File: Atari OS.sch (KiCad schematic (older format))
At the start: 3 parts, among them J51 OS Type, U7 27C512

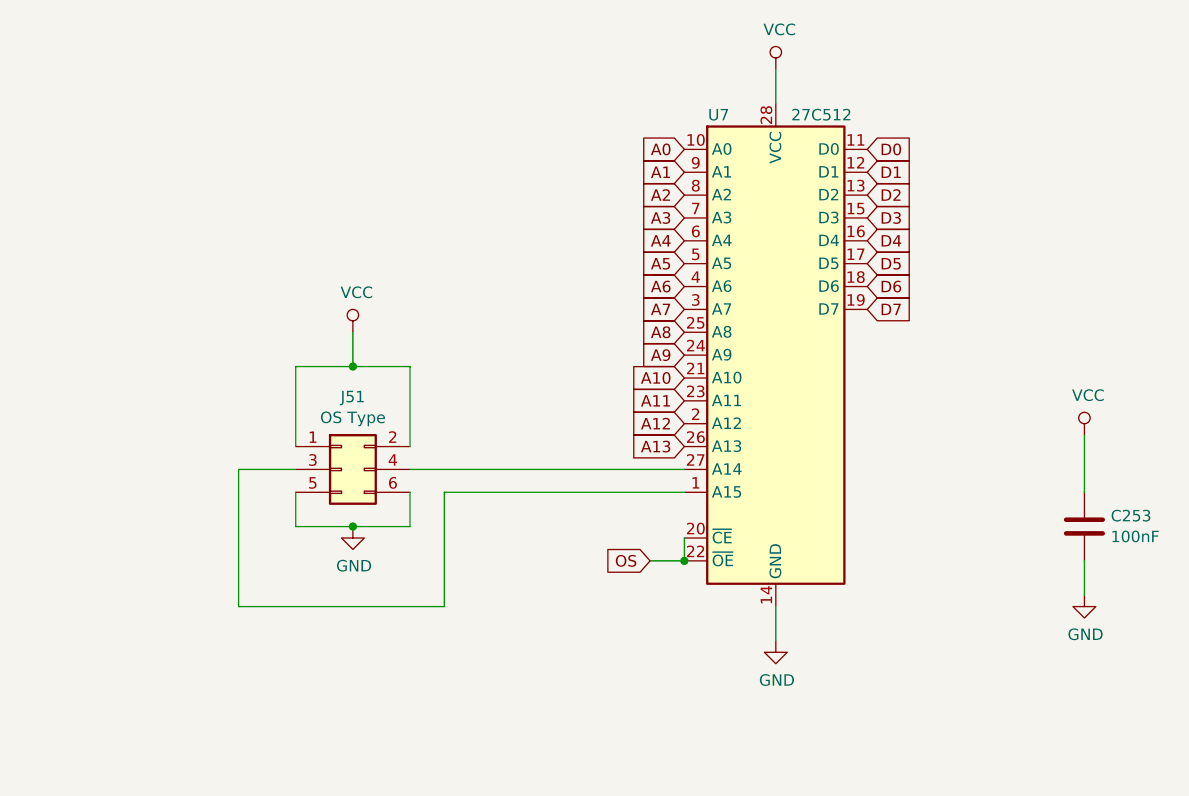
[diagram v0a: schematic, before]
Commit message: Track OS and Basic
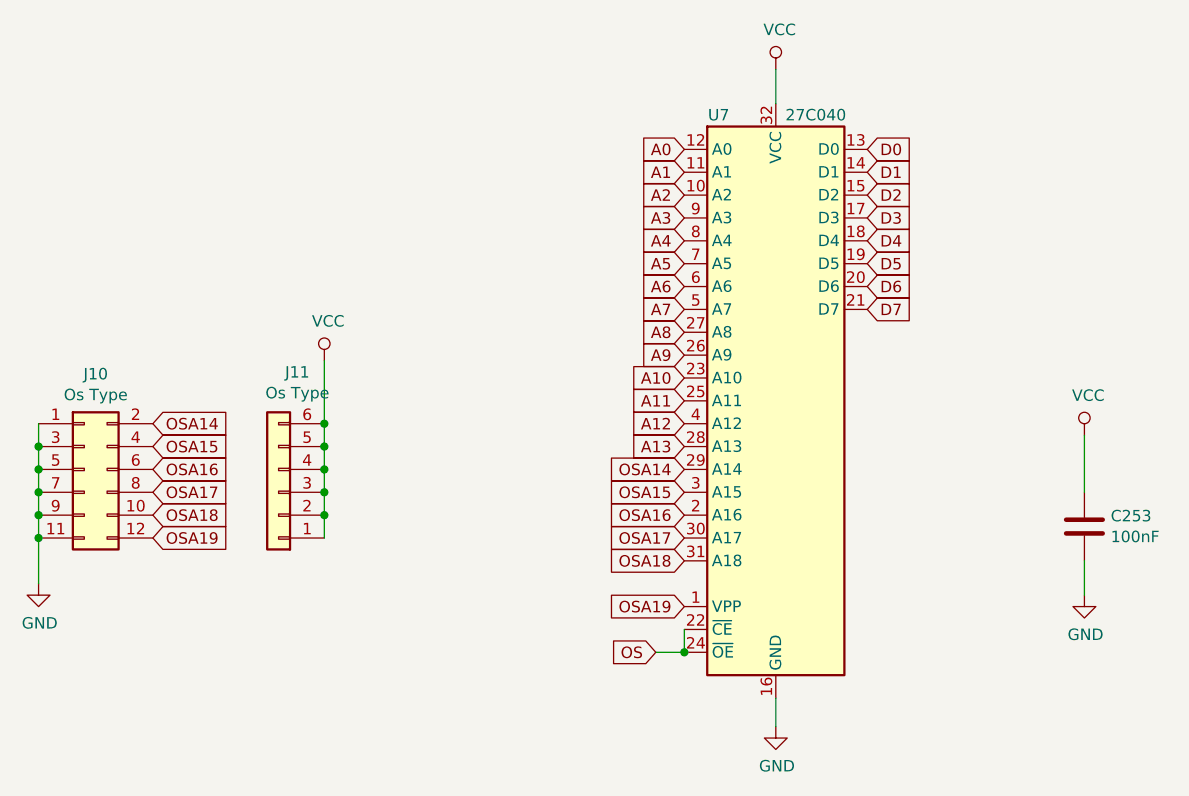
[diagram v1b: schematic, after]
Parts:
- removed J51: OS Type, Connector_PinHeader_2.54mm:PinHeader_2x03_P2.54mm_Vertical, symbol Connector_Generic:Conn_02x03_Odd_Even
- removed U7: 27C512, Package_DIP:DIP-28_W15.24mm_LongPads, symbol Memory_EPROM:27C512
- added J10: Os Type, Connector_PinHeader_2.54mm:PinHeader_2x06_P2.54mm_Vertical, symbol Connector_Generic:Conn_02x06_Odd_Even
- added J11: Os Type, Connector_PinHeader_2.54mm:PinHeader_1x06_P2.54mm_Vertical, symbol Connector_Generic:Conn_01x06
- added U7: 27C040, Package_DIP:DIP-32_W15.24mm_Socket_LongPads, symbol Memory_EPROM:27C040
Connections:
- net A0: now also U7.12 (A0)
- net A1: now also U7.11 (A1)
- net A10: now also U7.23 (A10)
- net A11: now also U7.25 (A11)
- net A12: now also U7.4 (A12)
- net A13: now also U7.28 (A13)
- net A2: now also U7.10 (A2)
- net A3: now also U7.9 (A3)
- net A4: now also U7.8 (A4)
- net A5: now also U7.7 (A5)
- net A6: now also U7.6 (A6)
- net A7: now also U7.5 (A7)
- net A8: now also U7.27 (A8)
- net A9: now also U7.26 (A9)
- net D0: now also U7.13 (D0)
- net D1: now also U7.14 (D1)
- net D2: now also U7.15 (D2)
- net D3: now also U7.17 (D3)
- net D4: now also U7.18 (D4)
- net D5: now also U7.19 (D5)
- net D6: now also U7.20 (D6)
- net D7: now also U7.21 (D7)
- net GND: now also J10.1 (Pin_1), J10.11 (Pin_11), J10.3 (Pin_3), J10.5 (Pin_5), J10.7 (Pin_7), J10.9 (Pin_9), U7.16 (GND)
- net OS: now also U7.22 (~CE), U7.24 (~OE)
- net VCC: now also J11.1 (Pin_1), J11.2 (Pin_2), J11.3 (Pin_3), J11.4 (Pin_4), J11.5 (Pin_5), J11.6 (Pin_6), U7.32 (VCC)
- new net OSA14: J10.2 (Pin_2), U7.29 (A14)
- new net OSA15: J10.4 (Pin_4), U7.3 (A15)
- new net OSA16: J10.6 (Pin_6), U7.2 (A16)
- new net OSA17: J10.8 (Pin_8), U7.30 (A17)
- new net OSA18: J10.10 (Pin_10), U7.31 (A18)
- new net OSA19: J10.12 (Pin_12), U7.1 (VPP)
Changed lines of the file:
@@
 $EndDescr
-$Comp
-L Memory_EPROM:27C512 U7
-U 1 1 5E64FA8C
-P 5850 3550
-F 0 "U7" H 5600 4600 50  0000 C CNN
-F 1 "27C512" H 6050 4600 50  0000 C CNN
-F 2 "Package_DIP:DIP-28_W15.24mm_LongPads" H 5850 3550 50  0001 C CNN
-F 3 "http://ww1.microchip.com/downloads/en/DeviceDoc/doc0015.pdf" H 5850 3550 50  0001 C CNN
-	1    5850 3550
-	1    0    0    -1
-$EndComp
 $Comp
 L power:VCC #PWR0185
@@
 L power:GND #PWR0186
 U 1 1 5E6514FE
-P 5850 4800
-F 0 "#PWR0186" H 5850 4550 50  0001 C CNN
-F 1 "GND" H 5855 4627 50  0000 C CNN
-F 2 "" H 5850 4800 50  0001 C CNN
-F 3 "" H 5850 4800 50  0001 C CNN
-	1    5850 4800
-	1    0    0    -1
-$EndComp
-Wire Wire Line
-	5850 4650 5850 4800
+P 5850 5175
+F 0 "#PWR0186" H 5850 4925 50  0001 C CNN
+F 1 "GND" H 5855 5002 50  0000 C CNN
+F 2 "" H 5850 5175 50  0001 C CNN
+F 3 "" H 5850 5175 50  0001 C CNN
+	1    5850 5175
+	1    0    0    -1
+$EndComp
 Text GLabel 6250 2650 2    50   Input ~ 0
 D0
@@
 A13
 $Comp
-L Connector_Generic:Conn_02x03_Odd_Even J51
-U 1 1 5E656178
-P 3950 4050
-F 0 "J51" H 4000 4367 50  0000 C CNN
-F 1 "OS Type" H 4000 4276 50  0000 C CNN
-F 2 "Connector_PinHeader_2.54mm:PinHeader_2x03_P2.54mm_Vertical" H 3950 4050 50  0001 C CNN
-F 3 "~" H 3950 4050 50  0001 C CNN
-	1    3950 4050
-	1    0    0    -1
-$EndComp
-$Comp
 L power:GND #PWR0187
 U 1 1 5E6585C8
-P 4000 4300
-F 0 "#PWR0187" H 4000 4050 50  0001 C CNN
-F 1 "GND" H 4005 4127 50  0000 C CNN
-F 2 "" H 4000 4300 50  0001 C CNN
-F 3 "" H 4000 4300 50  0001 C CNN
-	1    4000 4300
-	1    0    0    -1
-$EndComp
-Wire Wire Line
-	3750 4150 3750 4300
-Wire Wire Line
-	3750 4300 4000 4300
-Wire Wire Line
-	4250 4150 4250 4300
-Wire Wire Line
-	4250 4300 4000 4300
-Connection ~ 4000 4300
-Wire Wire Line
-	3750 3950 3750 3600
-Wire Wire Line
-	3750 3600 4000 3600
-Wire Wire Line
-	4250 3600 4250 3950
+P 2625 4550
+F 0 "#PWR0187" H 2625 4300 50  0001 C CNN
+F 1 "GND" H 2630 4377 50  0000 C CNN
+F 2 "" H 2625 4550 50  0001 C CNN
+F 3 "" H 2625 4550 50  0001 C CNN
+	1    2625 4550
+	1    0    0    -1
+$EndComp
 $Comp
 L power:VCC #PWR0188
 U 1 1 5E659359
-P 4000 3450
-F 0 "#PWR0188" H 4000 3300 50  0001 C CNN
-F 1 "VCC" H 4017 3623 50  0000 C CNN
-F 2 "" H 4000 3450 50  0001 C CNN
-F 3 "" H 4000 3450 50  0001 C CNN
-	1    4000 3450
-	1    0    0    -1
-$EndComp
-Wire Wire Line
-	4000 3450 4000 3600
-Connection ~ 4000 3600
-Wire Wire Line
-	4000 3600 4250 3600
-Wire Wire Line
-	5450 4050 4250 4050
-Wire Wire Line
-	5450 4150 4400 4150
-Wire Wire Line
-	4400 4150 4400 4650
-Wire Wire Line
-	4400 4650 3500 4650
-Wire Wire Line
-	3500 4650 3500 4050
-Wire Wire Line
-	3500 4050 3750 4050
-Wire Wire Line
-	5450 4350 5450 4450
-Text GLabel 5300 4450 0    50   Input ~ 0
+P 3875 3575
+F 0 "#PWR0188" H 3875 3425 50  0001 C CNN
+F 1 "VCC" H 3892 3748 50  0000 C CNN
+F 2 "" H 3875 3575 50  0001 C CNN
+F 3 "" H 3875 3575 50  0001 C CNN
+	1    3875 3575
+	1    0    0    -1
+$EndComp
+Text GLabel 5325 4850 0    50   Input ~ 0
 OS
-Wire Wire Line
-	5450 4450 5300 4450
-Connection ~ 5450 4450
 $Comp
 L Device:C C253
@@
 Wire Wire Line
 	7200 3900 7200 4150
+$Comp
+L Memory_EPROM:27C040 U7
+U 1 1 5FC01AF4
+P 5850 3750
+F 0 "U7" H 5600 5000 50  0000 C CNN
+F 1 "27C040" H 6025 5000 50  0000 C CNN
+F 2 "Package_DIP:DIP-32_W15.24mm_Socket_LongPads" H 5850 3750 50  0001 C CNN
+F 3 "http://ww1.microchip.com/downloads/en/devicedoc/doc0189.pdf" H 5850 3750 50  0001 C CNN
+	1    5850 3750
+	1    0    0    -1
+$EndComp
+Wire Wire Line
+	5450 4750 5450 4850
+Wire Wire Line
+	5450 4850 5325 4850
+Connection ~ 5450 4850
+Wire Wire Line
+	5850 5050 5850 5175
+$Comp
+L Connector_Generic:Conn_02x06_Odd_Even J10
+U 1 1 5FC22FF9
+P 2825 4050
+F 0 "J10" H 2875 4467 50  0000 C CNN
+F 1 "Os Type" H 2875 4376 50  0000 C CNN
+F 2 "Connector_PinHeader_2.54mm:PinHeader_2x06_P2.54mm_Vertical" H 2825 4050 50  0001 C CNN
+F 3 "~" H 2825 4050 50  0001 C CNN
+	1    2825 4050
+	1    0    0    -1
+$EndComp
+$Comp
+L Connector_Generic:Conn_01x06 J11
+U 1 1 5FC26BAD
+P 3675 4150
+F 0 "J11" H 3593 3625 50  0000 C CNN
+F 1 "Os Type" H 3593 3716 50  0000 C CNN
+F 2 "Connector_PinHeader_2.54mm:PinHeader_1x06_P2.54mm_Vertical" H 3675 4150 50  0001 C CNN
+F 3 "~" H 3675 4150 50  0001 C CNN
+	1    3675 4150
+	-1   0    0    1
+$EndComp
+Wire Wire Line
+	2625 3850 2625 3950
+Wire Wire Line
+	2625 3950 2625 4050
+Connection ~ 2625 3950
+Wire Wire Line
+	2625 4050 2625 4150
+Connection ~ 2625 4050
+Wire Wire Line
+	2625 4150 2625 4250
+Connection ~ 2625 4150
+Wire Wire Line
+	2625 4250 2625 4350
+Connection ~ 2625 4250
+Wire Wire Line
+	2625 4350 2625 4550
+Connection ~ 2625 4350
+Wire Wire Line
+	3875 3850 3875 3950
+Wire Wire Line
+	3875 4050 3875 3950
+Connection ~ 3875 3950
+Wire Wire Line
+	3875 4150 3875 4050
+Connection ~ 3875 4050
+Connection ~ 3875 4150
+Wire Wire Line
+	3875 4150 3875 4250
+Wire Wire Line
+	3875 4350 3875 4250
+Connection ~ 3875 4250
+Wire Wire Line
+	3875 3850 3875 3575
+Connection ~ 3875 3850
+Text GLabel 5450 4050 0    50   Input ~ 0
+OSA14
+Text GLabel 5450 4150 0    50   Input ~ 0
+OSA15
+Text GLabel 5450 4250 0    50   Input ~ 0
+OSA16
+Text GLabel 5450 4450 0    50   Input ~ 0
+OSA18
+Text GLabel 5450 4350 0    50   Input ~ 0
+OSA17
+Text GLabel 3125 3850 2    50   Input ~ 0
+OSA14
+Text GLabel 3125 3950 2    50   Input ~ 0
+OSA15
+Text GLabel 3125 4050 2    50   Input ~ 0
+OSA16
+Text GLabel 3125 4150 2    50   Input ~ 0
+OSA17
+Text GLabel 3125 4250 2    50   Input ~ 0
+OSA18
+Text GLabel 5450 4650 0    50   Input ~ 0
+OSA19
+Text GLabel 3125 4350 2    50   Input ~ 0
+OSA19
 $EndSCHEMATC
